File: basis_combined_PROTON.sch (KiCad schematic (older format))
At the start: 186 parts, among them J3 USB_B_Micro, J4 USB_B_Micro, SW1 Rotary_Encoder_Switch, SW2 Rotary_Encoder_Switch, SW3 Rotary_Encoder_Switch, SW4 SW_Push, SW5 SW_Push, U1 ATmega32U4-AU, U2 ATmega32U4-AU, Y1 Crystal_GND24_Small, Y2 Crystal_GND24_Small

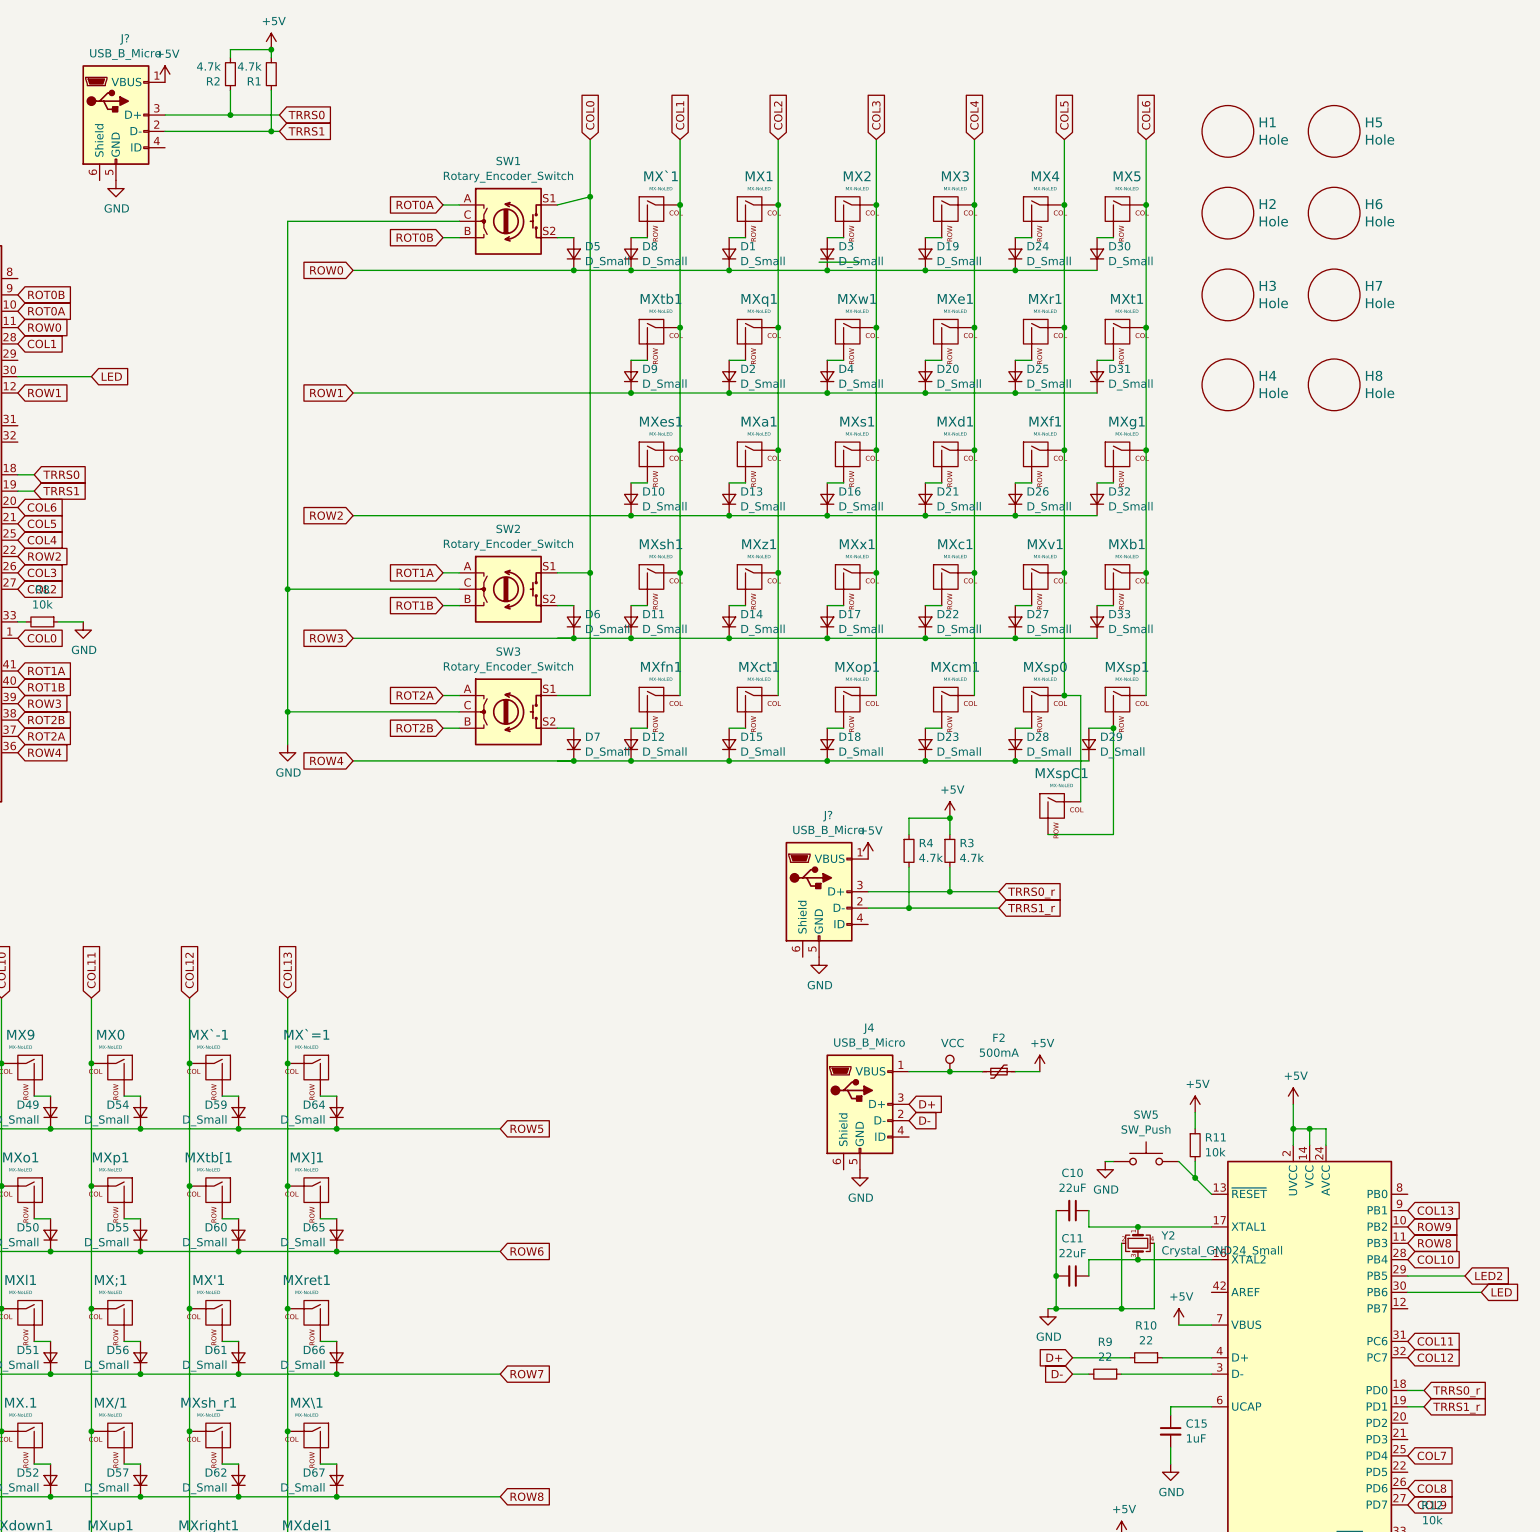
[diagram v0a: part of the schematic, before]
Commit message: version sent to pcb manu
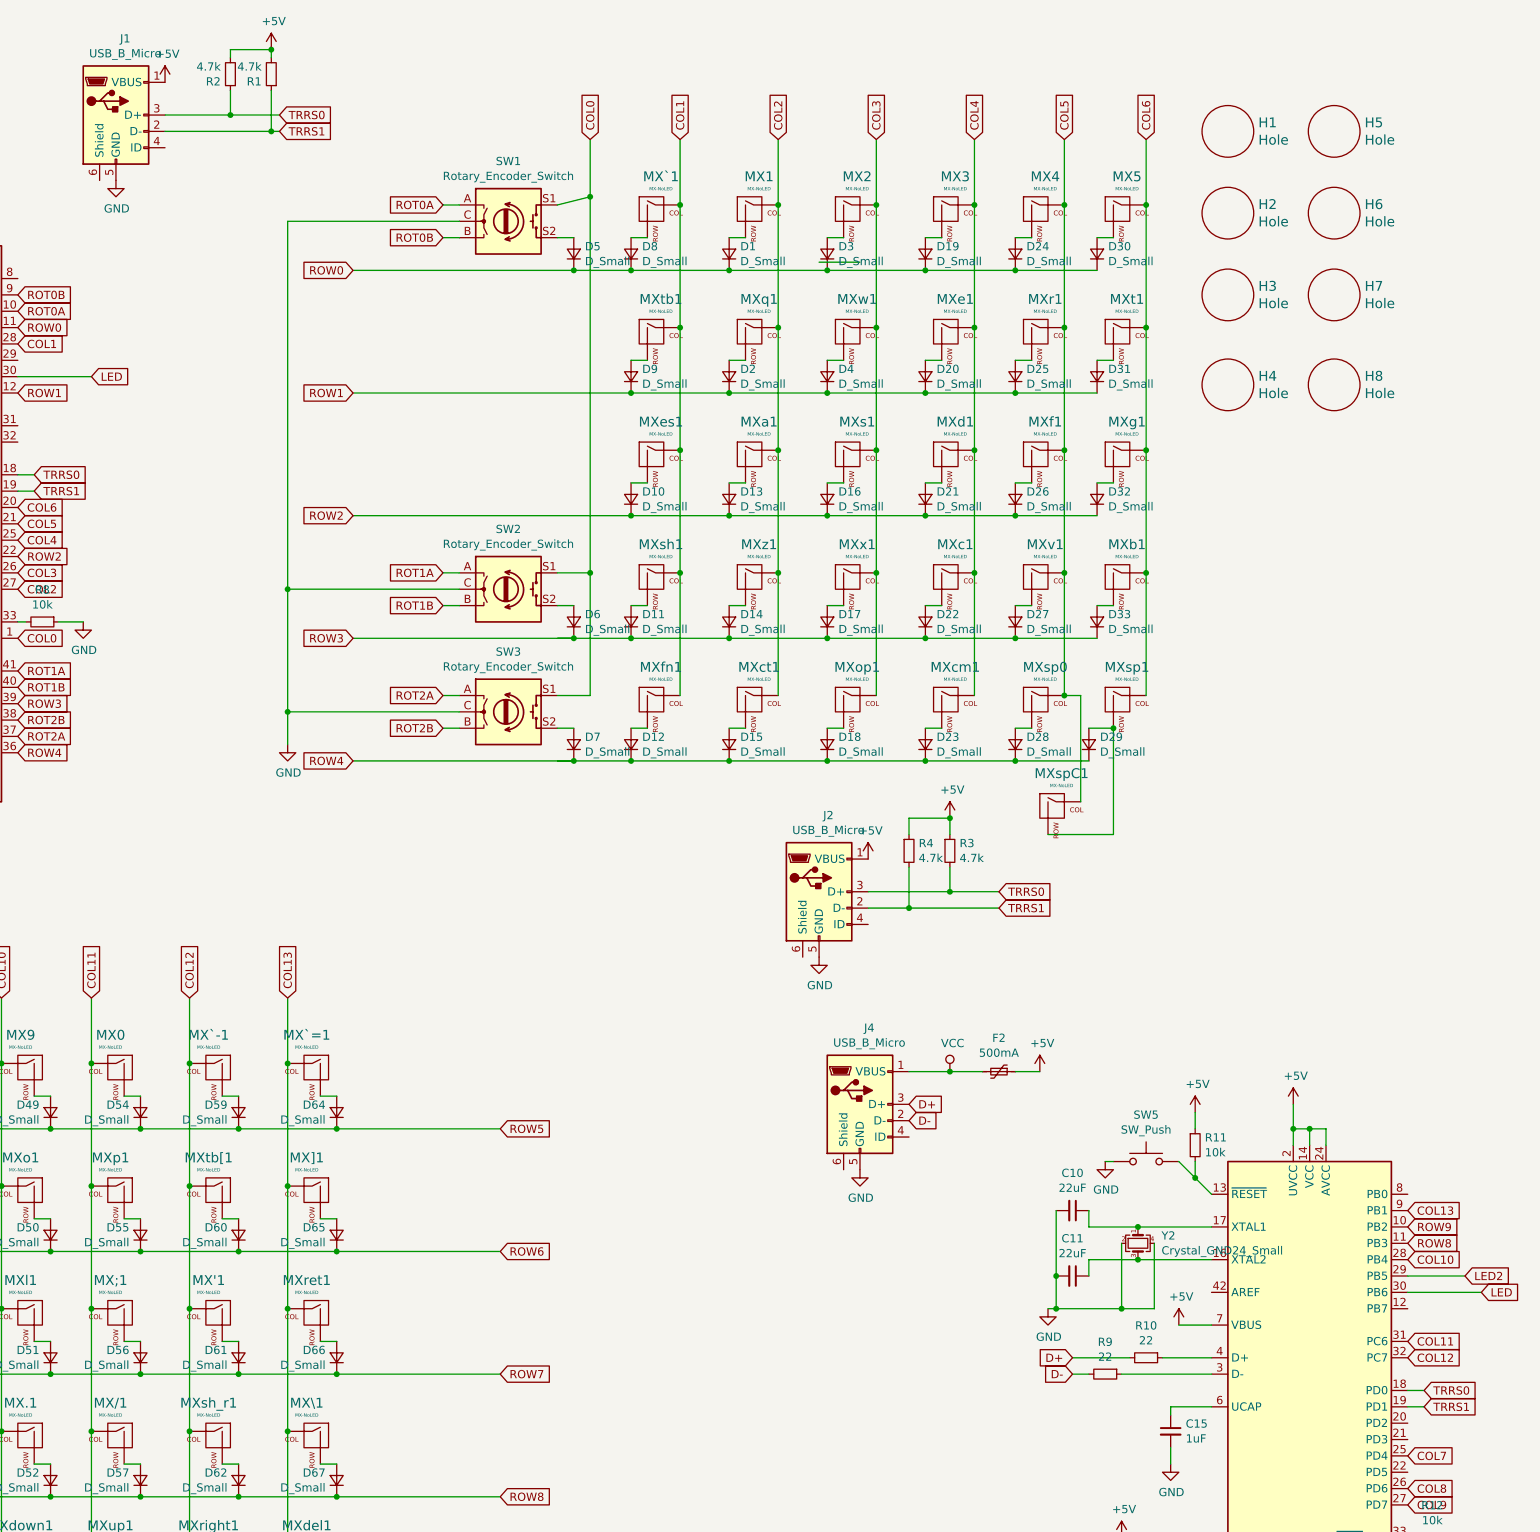
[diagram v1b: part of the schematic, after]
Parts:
- gave numbers to parts that had none: 2
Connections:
- net TRRS0_r is gone; now on net TRRS0: J2.3 (D+), R3.2, U2.18 (PD0)
- net TRRS1_r is gone; now on net TRRS1: J2.2 (D-), R4.2, U2.19 (PD1)
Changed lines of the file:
@@
 $EndComp
 Text GLabel 8850 5850 2    50   Input ~ 0
-TRRS1_r
+TRRS1
 Text GLabel 8850 5750 2    50   Input ~ 0
-TRRS0_r
+TRRS0
 Wire Wire Line
 	8050 5750 8550 5750
@@
 ROW5
 Text GLabel 11450 8900 2    50   Input ~ 0
-TRRS1_r
+TRRS1
 Text GLabel 11450 8800 2    50   Input ~ 0
-TRRS0_r
+TRRS0
 $Comp
 L power:+5V #PWR0105
@@
 Connection ~ 8550 6850
 $Comp
-L Connector:USB_B_Micro J?
+L Connector:USB_B_Micro J2
 U 1 1 6171A6A9
 P 7750 5750
-F 0 "J?" H 7807 6217 50  0000 C CNN
+F 0 "J2" H 7807 6217 50  0000 C CNN
 F 1 "USB_B_Micro" H 7807 6126 50  0000 C CNN
 F 2 "Connector_USB:USB_Micro-B_Molex_47346-0001" H 7900 5700 50  0001 C CNN
@@
 $EndComp
 $Comp
-L Connector:USB_B_Micro J?
+L Connector:USB_B_Micro J1
 U 1 1 6171CFCD
 P 3450 1000
-F 0 "J?" H 3507 1467 50  0000 C CNN
+F 0 "J1" H 3507 1467 50  0000 C CNN
 F 1 "USB_B_Micro" H 3507 1376 50  0000 C CNN
 F 2 "Connector_USB:USB_Micro-B_Molex_47346-0001" H 3600 950 50  0001 C CNN

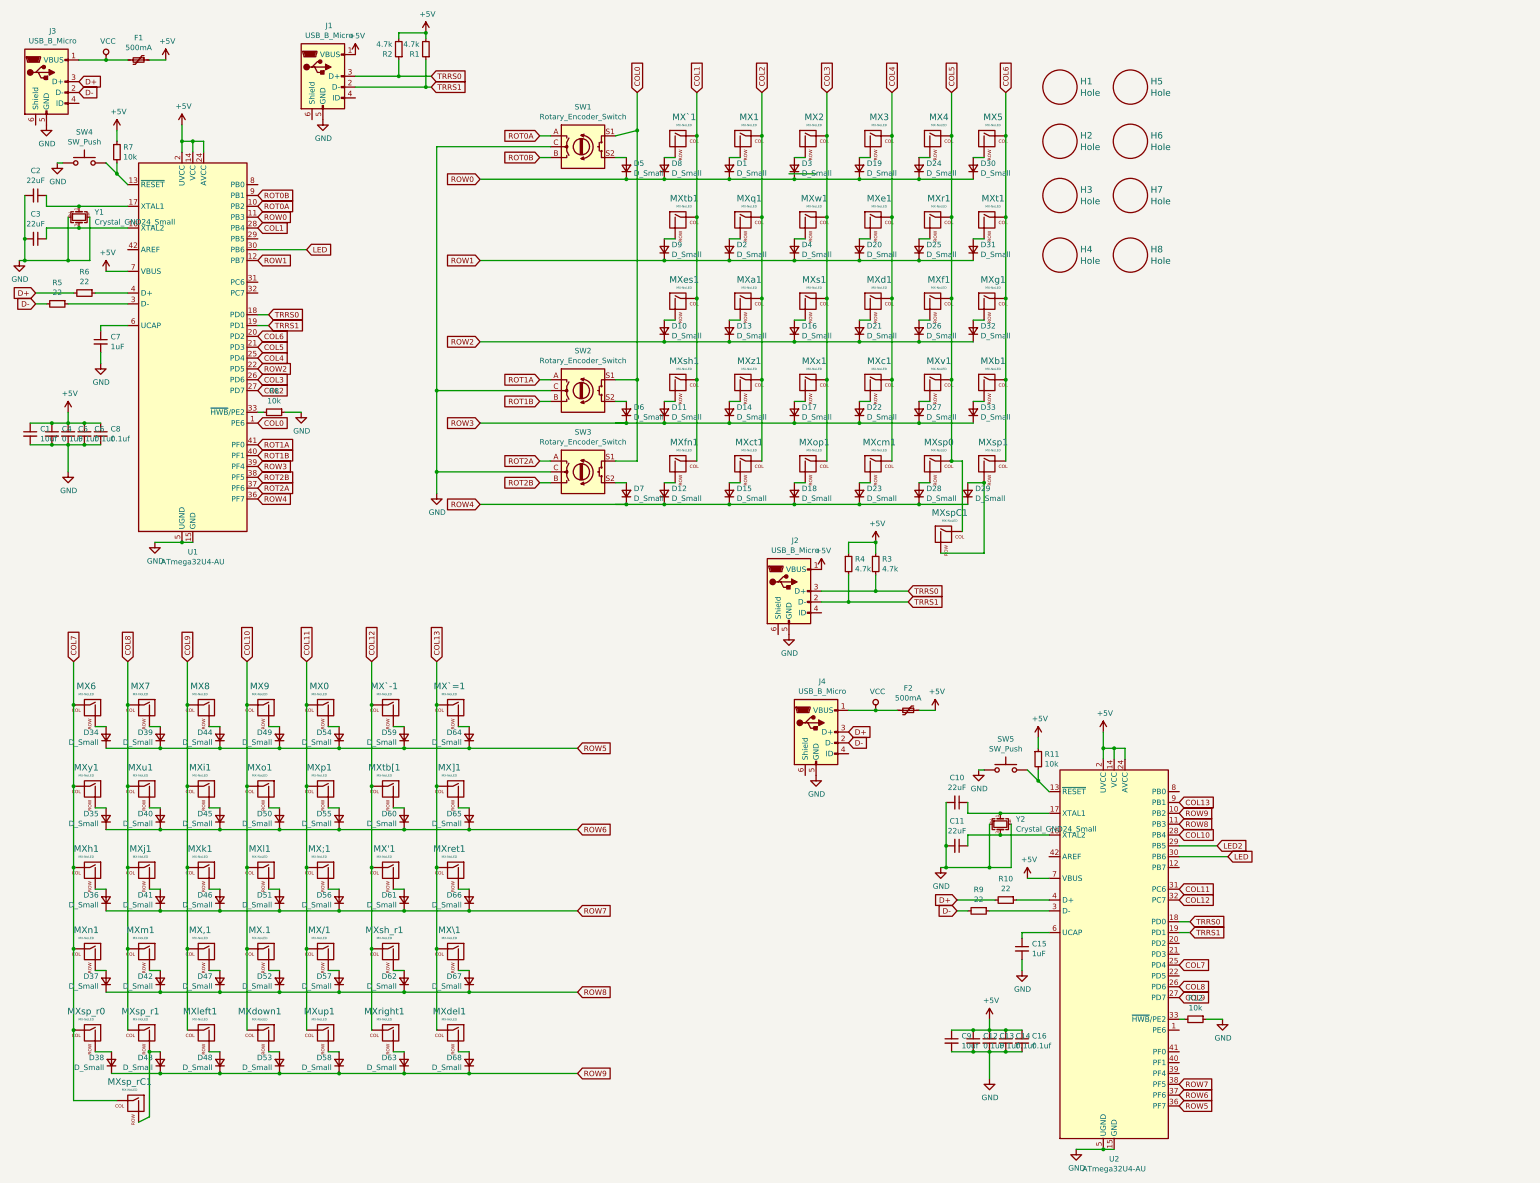
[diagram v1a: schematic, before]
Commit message: Added a bunch of cleanup etc
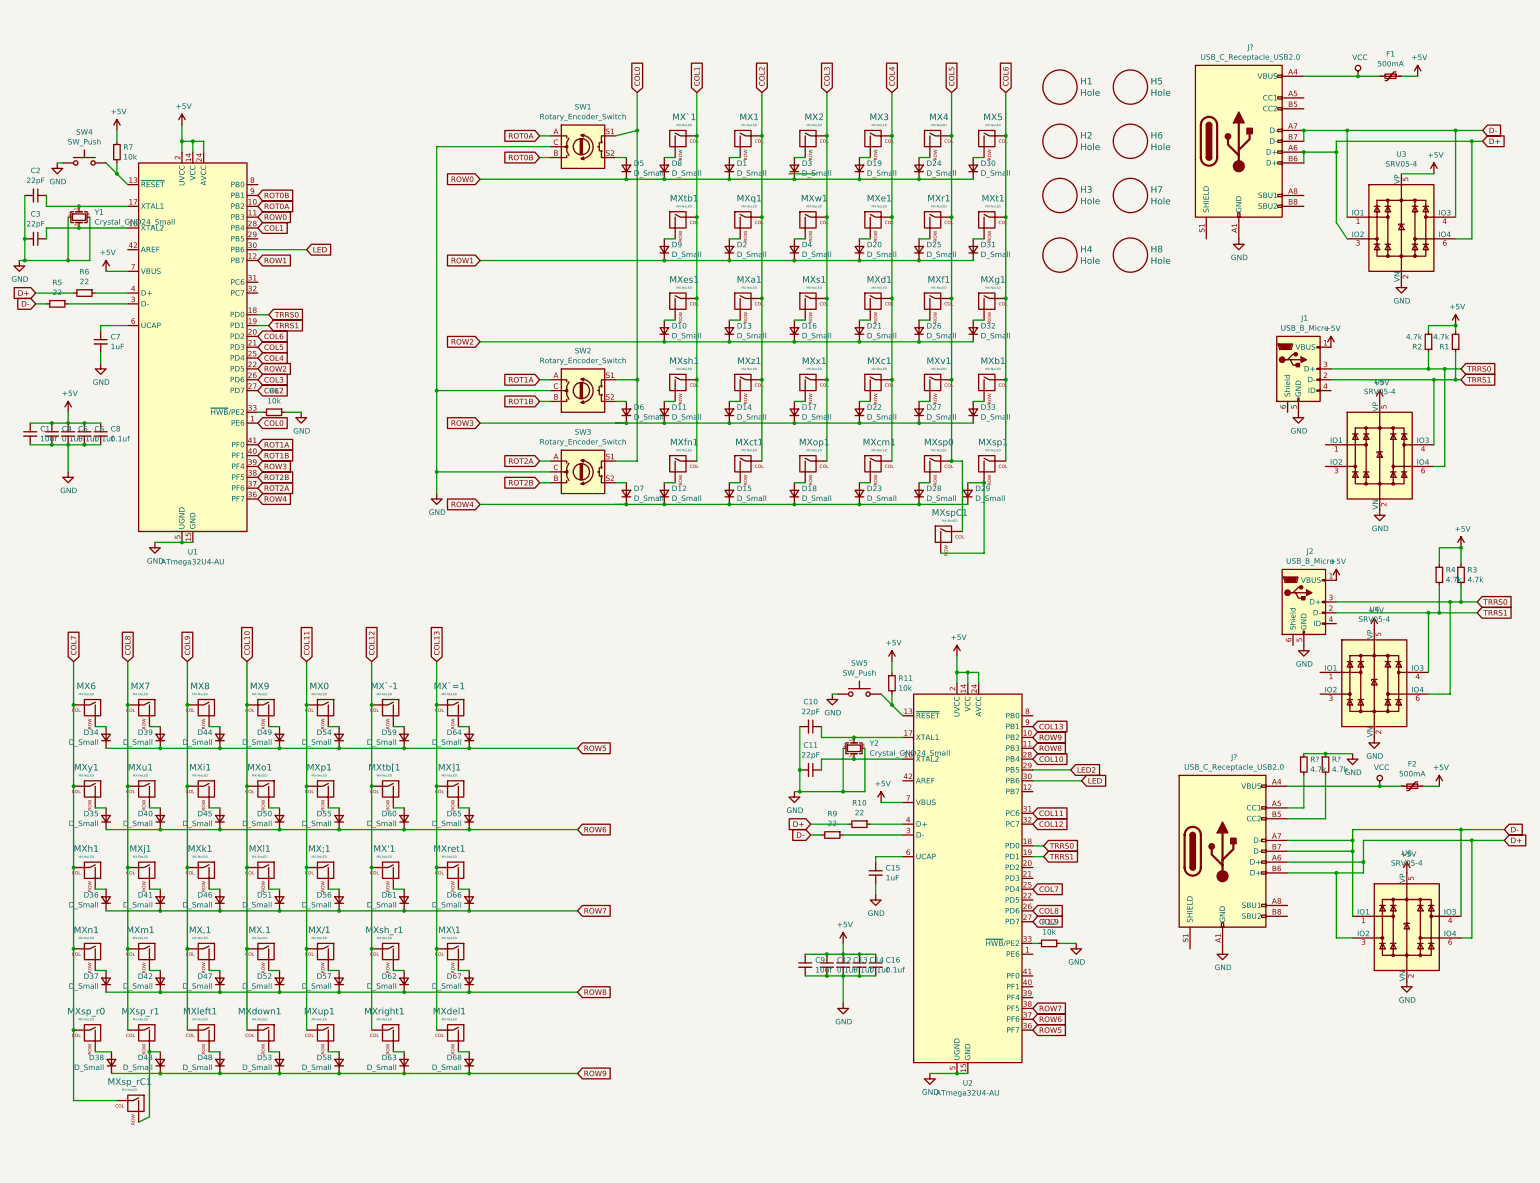
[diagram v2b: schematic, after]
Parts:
- removed J3, J4: USB_B_Micro, Connector_USB:USB_Micro-B_Molex_47346-0001, symbol Connector:USB_B_Micro
- added J? (x2): USB_C_Receptacle_USB2.0, symbol Connector:USB_C_Receptacle_USB2.0
- added R? (x2): 4.7k, Resistor_SMD:R_0805_2012Metric, symbol Device:R_Small
- added U3, U4, U5, U6: SRV05-4, Package_TO_SOT_SMD:SOT-23-6, symbol Power_Protection:SRV05-4
- C10, C11, C2, C3: value 22uF -> 22pF
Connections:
- net +5V: now also U3.5 (VP), U4.5 (VP), U5.5 (VP), U6.5 (VP)
- net D+: now also J?.A6 (D+), J?.A6 (D+), J?.B6 (D+), J?.B6 (D+), U3.3 (IO2), U3.6 (IO4), U6.3 (IO2), U6.6 (IO4)
- net D-: now also J?.A7 (D-), J?.A7 (D-), J?.B7 (D-), J?.B7 (D-), U3.1 (IO1), U3.4 (IO3), U6.1 (IO1), U6.4 (IO3)
- net GND: now also J?.A1 (GND), J?.A1 (GND), J?.A12 (GND), J?.A12 (GND), J?.B1 (GND), J?.B1 (GND), J?.B12 (GND), J?.B12 (GND), R?.1, R?.1, U3.2 (VN), U4.2 (VN), U5.2 (VN), U6.2 (VN)
- net TRRS0: now also U4.6 (IO4), U5.6 (IO4)
- net TRRS1: now also U4.4 (IO3), U5.4 (IO3)
- net VCC: now also J?.A4 (VBUS), J?.A4 (VBUS), J?.A9 (VBUS), J?.A9 (VBUS), J?.B4 (VBUS), J?.B4 (VBUS), J?.B9 (VBUS), J?.B9 (VBUS)
- new net: J?.A5 (CC1), R?.2
- new net: J?.B5 (CC2), R?.2
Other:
- moved on the sheet: C10, C11, C12, C13, C14, C15, C16, C9, F1, F2, J1, J2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
